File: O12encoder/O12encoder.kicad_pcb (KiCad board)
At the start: 2 copper layers, 14 x 14 mm, 17 parts, among them J1 Conn_01x06_Pin, J2 Conn_01x06_Pin, J3 Conn_01x06_Pin, J4 Conn_01x06_Pin, J5 JST_SM02B-SRSS-TB(LF)(SN), J6 Conn_01x06_Pin, J7 Conn_01x06_Pin, J8 Conn_01x06_Pin, U1 MA702GQ-P, U2 STM32L011F4Ux, U3 THVD1420DRLR

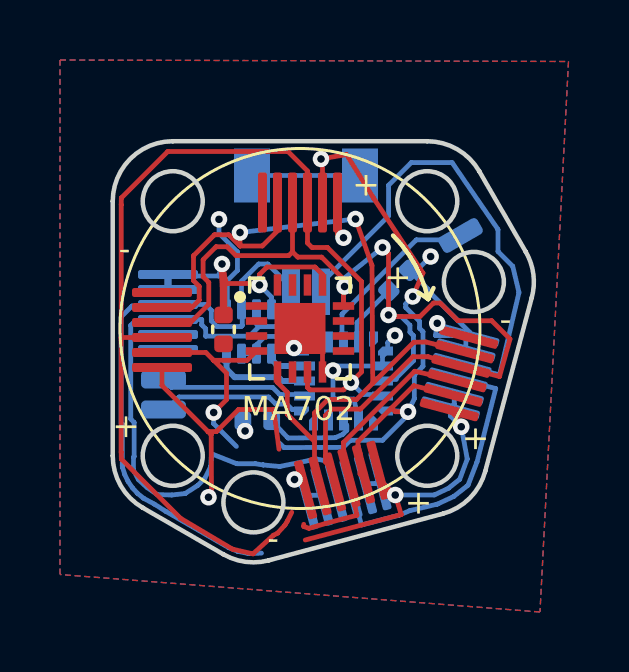
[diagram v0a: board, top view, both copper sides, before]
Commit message: done? added silkscreen and pa0 breakout
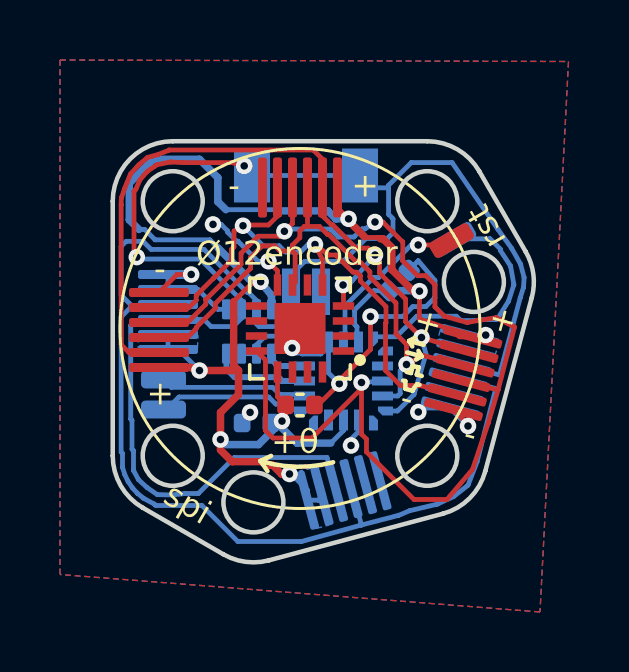
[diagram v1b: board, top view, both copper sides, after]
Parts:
- removed J3: Conn_01x06_Pin, O32controller:FFC_0.5mm_6p
- added TP4: TestPoint, O32controller:TestPoint_Pad_Rect, B.Cu at (55.1, 47.0)
- TP1: moved to F.Cu
- moved C1 3.59 mm to (50.0, 52.5), turned to 0 degrees
- moved J6 2.50 mm to (45.6, 48.2), turned to 180 degrees
- moved J7 2.50 mm to (55.0, 52.6), turned to -15 degrees
- moved J8 2.50 mm to (52.7, 55.1), turned to 105 degrees
- moved J4 2.46 mm to (55.1, 52.7), turned to 165 degrees
- moved J2 0.50 mm to (48.8, 45.3)
- moved TP1 0.34 mm to (55.0, 47.1)
- moved J1 0.10 mm to (45.3, 48.8)
- moved C2 0.08 mm to (48.5, 53.1)
- turned U1 to 180 degrees
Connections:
- J5 pad S1: unconnected-(J5-Shield-PadS1) -> /RS485_A
- J5 pad S2: unconnected-(J5-Shield-PadS1) -> /RS485_A
- U2 pad 2: unconnected-(U2-PC15-Pad2) -> GND
- U2 pad 6: GND -> unconnected-(U2-PA1-Pad6)
- U2 pad 7: GND -> unconnected-(U2-PA4-Pad7)
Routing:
- net /SPI_MISO: track 44.8 -> 19.2 mm
- net /RS485_A: track 29.2 -> 50.9 mm, vias 0 -> 2
- net +3.3V: track 37.9 -> 50.7 mm, vias 6 -> 8
- net /~{MAG2_CS}: track 27.4 -> 18.6 mm
- net /ADC_IN0/WKUP: track 0.00 -> 8.72 mm
- net /SPI_SCLK: track 32.9 -> 38.0 mm
- net GND: track 18.9 -> 23.9 mm, vias 8 -> 10
- net unconnected-(J5-Shield-PadS1): track 3.60 -> 0.00 mm
- net /SPI_MOSI: track 30.6 -> 28.5 mm, vias 4 -> 3
- net /RS485_B: track 38.8 -> 37.4 mm
- net /NRST: track 6.04 -> 5.67 mm, vias 0 -> 1
- added copper zone on B.Cu, net +3.3V
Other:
- board text added: "+θ"
- board text added: "a"
- board text added: "b"
- board text added: "clk"
- board text added: "io"
- board text added: "pa0"
- board text added: "rs485"
- board text added: "rst"
- board text added: "spi"
- board text added: "Ø12encoder"
- board text removed: "MA702"
